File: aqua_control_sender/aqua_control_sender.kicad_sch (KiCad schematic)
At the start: 37 parts, among them J1 USB_C, J4 Conn_01x03, J5 Conn_01x03, SW1 RESET, SW2 BOOT, U1 ESP32-S3-WROOM-1, U2 LM1117-3.3, U3 RA-02_LORA

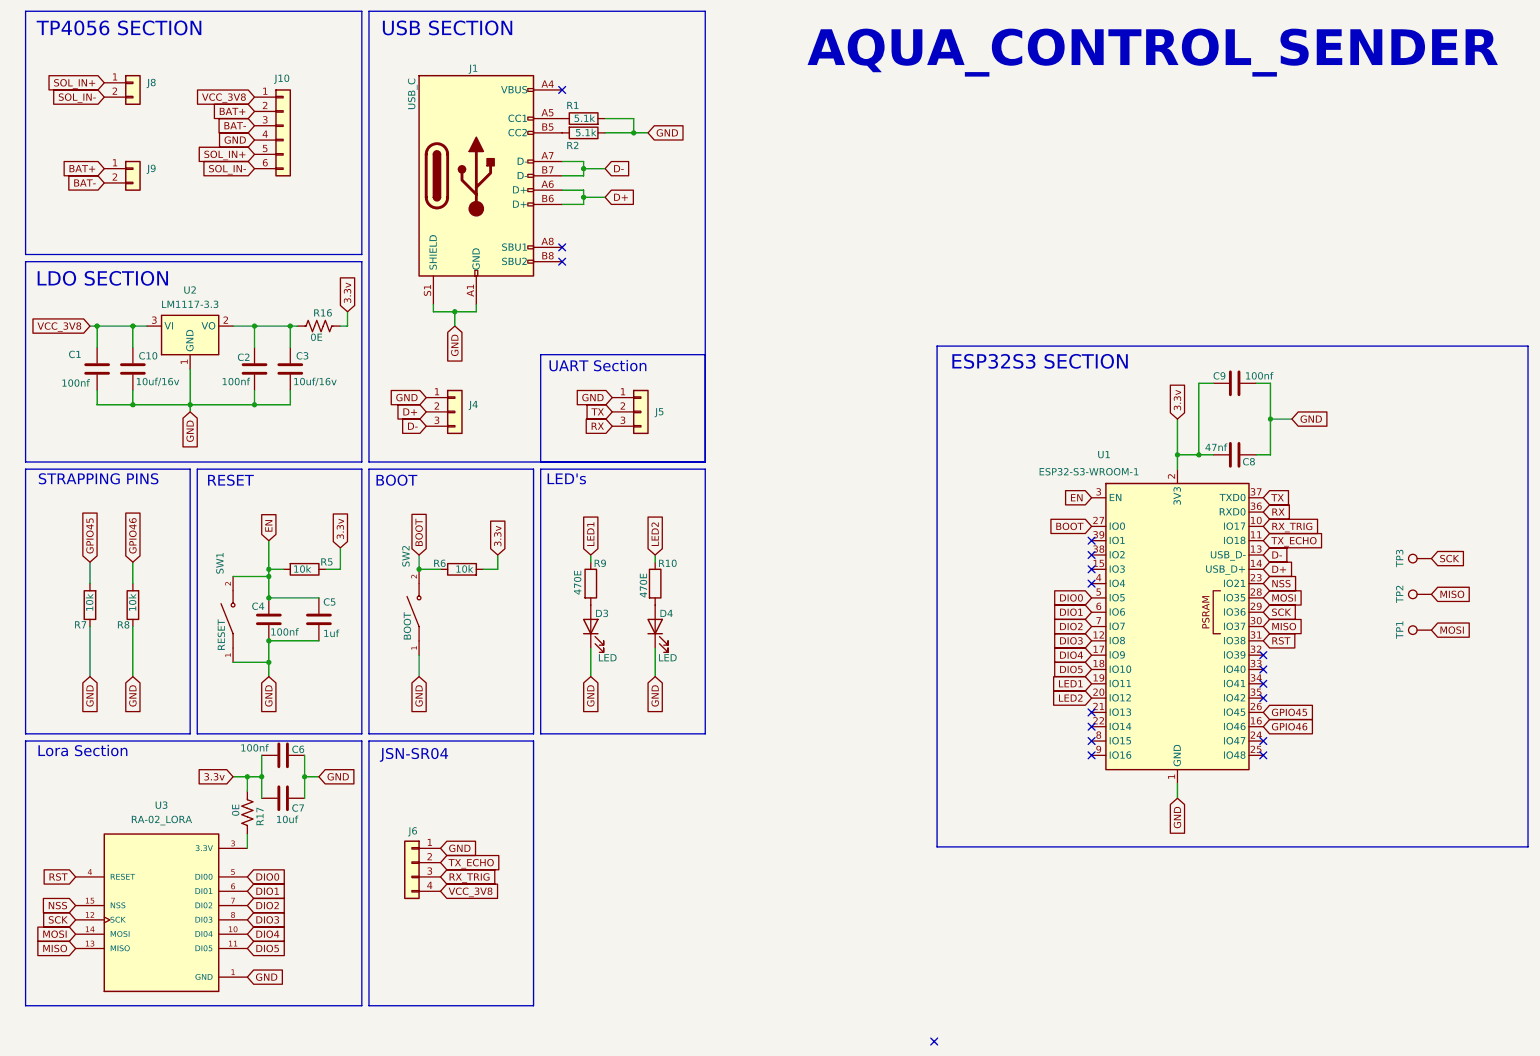
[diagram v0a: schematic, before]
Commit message: sender board complete
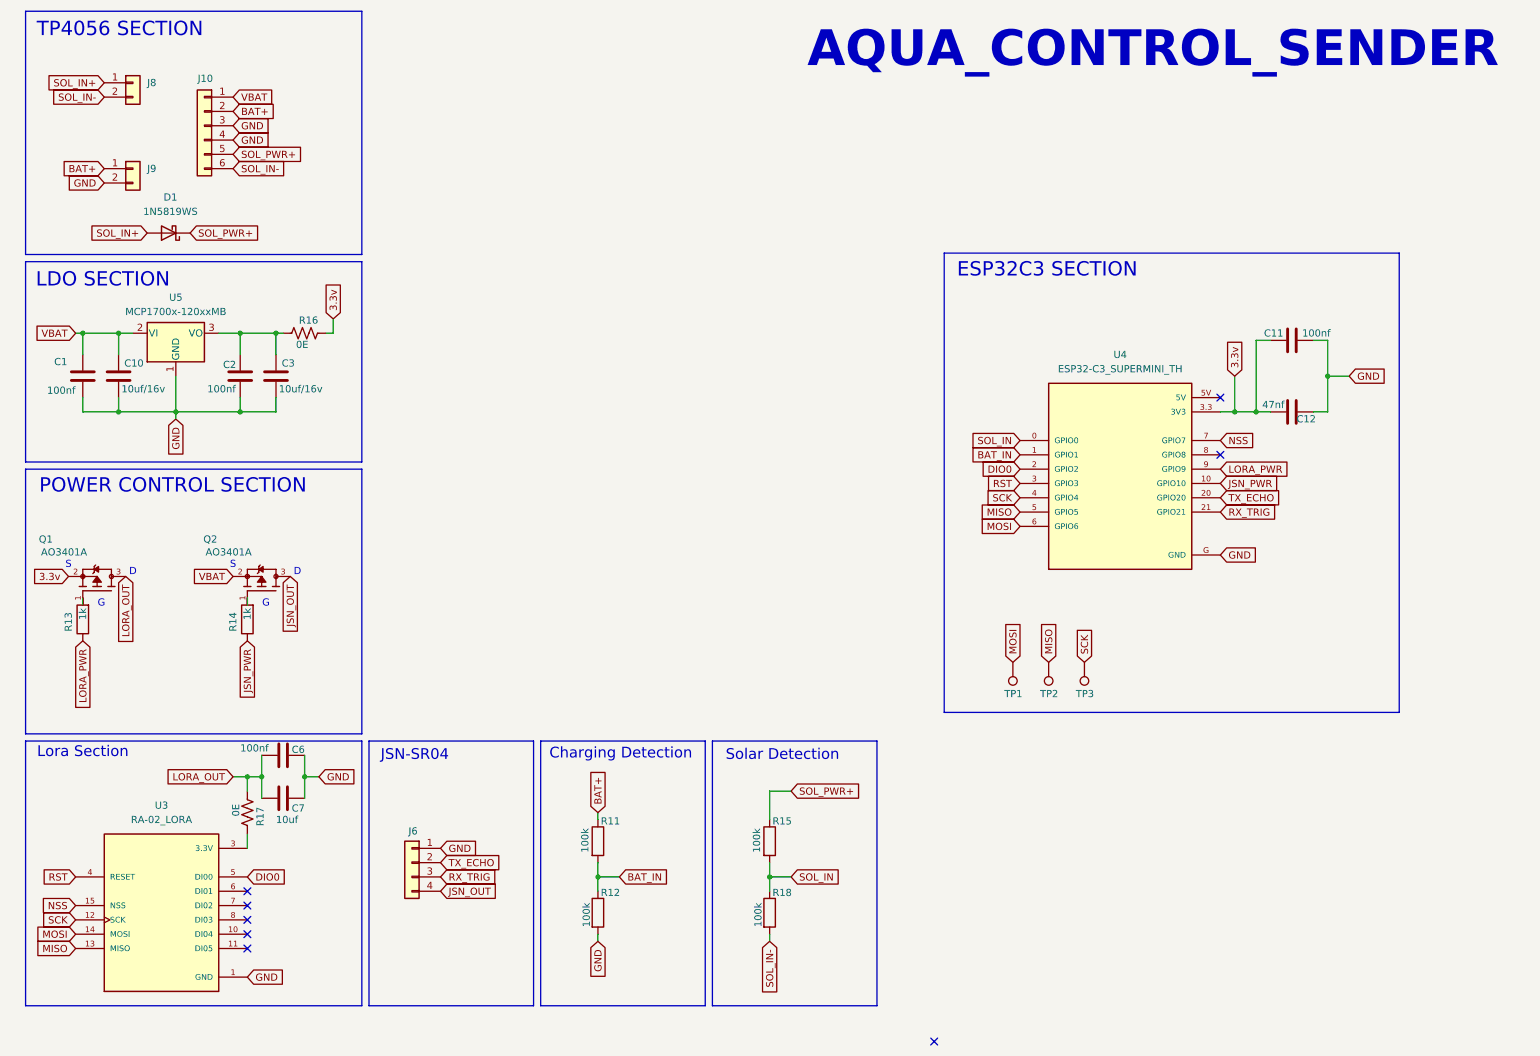
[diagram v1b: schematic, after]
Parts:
- removed C4, C9: 100nf, Capacitor_SMD:C_0805_2012Metric_Pad1.18x1.45mm_HandSolder, symbol Device:C
- removed C5: 1uf, Capacitor_SMD:C_0805_2012Metric_Pad1.18x1.45mm_HandSolder, symbol Device:C
- removed C8: 47nf, Capacitor_SMD:C_0805_2012Metric_Pad1.18x1.45mm_HandSolder, symbol Device:C
- removed D3, D4: LED, LED_SMD:LED_1206_3216Metric_Pad1.42x1.75mm_HandSolder, symbol Device:LED
- removed J1: USB_C, Connector_USB:USB_C_Receptacle_GCT_USB4110, symbol Connector:USB_C_Receptacle_USB2.0_16P
- removed J4, J5: Conn_01x03, Connector_PinSocket_2.54mm:PinSocket_1x03_P2.54mm_Vertical, symbol Connector_Generic:Conn_01x03
- removed R1, R2: 5.1k, Resistor_SMD:R_0805_2012Metric_Pad1.20x1.40mm_HandSolder, symbol Device:R
- removed R10, R9: 470E, Resistor_SMD:R_0805_2012Metric_Pad1.20x1.40mm_HandSolder, symbol Device:R
- removed R5, R6, R7, R8: 10k, Resistor_SMD:R_0805_2012Metric_Pad1.20x1.40mm_HandSolder, symbol Device:R
- removed SW1: RESET, Button_Switch_THT:SW_DIP_SPSTx01_Slide_6.7x4.1mm_W7.62mm_P2.54mm_LowProfile, symbol TS09-63-25-WT-160-SMT-TR:TS09-63-25-WT-160-SMT-TR
- removed SW2: BOOT, Button_Switch_THT:SW_DIP_SPSTx01_Slide_6.7x4.1mm_W7.62mm_P2.54mm_LowProfile, symbol TS09-63-25-WT-160-SMT-TR:TS09-63-25-WT-160-SMT-TR
- removed U1: ESP32-S3-WROOM-1, RF_Module:ESP32-S3-WROOM-1, symbol RF_Module:ESP32-S3-WROOM-1
- removed U2: LM1117-3.3, Package_TO_SOT_SMD:SOT-223-3_TabPin2, symbol Regulator_Linear:AMS1117-3.3
- added C11: 100nf, Capacitor_SMD:C_0805_2012Metric_Pad1.18x1.45mm_HandSolder, symbol Device:C
- added C12: 47nf, Capacitor_SMD:C_0805_2012Metric_Pad1.18x1.45mm_HandSolder, symbol Device:C
- added D1: 1N5819WS, Diode_SMD:D_SOD-323, symbol Diode:1N5819WS
- added Q1, Q2: AO3401A, mosfet:SOT23-3, symbol AO3401A:AO3401A
- added R11, R12, R15, R18: 100k, Resistor_SMD:R_0805_2012Metric_Pad1.20x1.40mm_HandSolder, symbol Device:R
- added R13, R14: 1k, Resistor_SMD:R_0805_2012Metric_Pad1.20x1.40mm_HandSolder, symbol Device:R
- added U4: ESP32-C3_SUPERMINI_TH, esp32c3:MODULE_ESP32-C3_SUPERMINI_TH, symbol ESP32-C3_SUPERMINI_TH:ESP32-C3_SUPERMINI_TH
- added U5: MCP1700x-120xxMB, Package_TO_SOT_SMD:SOT-89-3, symbol Regulator_Linear:MCP1700x-120xxMB
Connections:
- net BAT- is gone; now on net GND: J10.3 (Pin_3), J9.2 (Pin_2)
- net 3.3v: now also C11.1, C12.1, Q1.2, U4.3.3 (3V3); no longer C6.2, C7.2, R17.2
- net BAT+: now also R11.1
- net DIO0: now also U4.2 (GPIO2)
- net GND: now also C11.2, C12.2, R12.2, U4.G (GND), U5.1 (GND)
- net MISO: now also U4.5 (GPIO5)
- net MOSI: now also U4.6 (GPIO6)
- net NSS: now also U4.7 (GPIO7)
- net RST: now also U4.3 (GPIO3)
- net RX_TRIG: now also U4.21 (GPIO21)
- net SCK: now also U4.4 (GPIO4)
- net SOL_IN+: now also D1.2 (A); no longer J10.5 (Pin_5)
- net SOL_IN-: now also R18.2
- net TX_ECHO: now also U4.20 (GPIO20)
- net at C2.1, C3.1, R16.2: now also U5.3 (VO)
- net DIO1: no longer names the net of U3.6 (DI01)
- net DIO2: no longer names the net of U3.7 (DI02)
- net DIO3: no longer names the net of U3.8 (DI03)
- net DIO4: no longer names the net of U3.10 (DI04)
- net DIO5: no longer names the net of U3.11 (DI05)
- net VCC_3V8 renamed VBAT
- net VBAT: now also Q2.2, U5.2 (VI); no longer J6.4 (Pin_4)
- new net: Q1.1, R13.2
- new net: Q2.1, R14.2
- new net BAT_IN: R11.2, R12.1, U4.1 (GPIO1)
- new net JSN_OUT: J6.4 (Pin_4), Q2.3
- new net JSN_PWR: R14.1, U4.10 (GPIO10)
- new net LORA_OUT: C6.2, C7.2, Q1.3, R17.2
- new net LORA_PWR: R13.1, U4.9 (GPIO9)
- new net SOL_IN: R15.2, R18.1, U4.0 (GPIO0)
- new net SOL_PWR+: D1.1 (K), J10.5 (Pin_5), R15.1
- no-connect marks 18 -> 8
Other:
- note added: "Charging Detection"
- note added: "D"
- note added: "ESP32C3 SECTION"
- note added: "G"
- note added: "POWER CONTROL SECTION"
- note added: "S"
- note added: "Solar Detection"
- note removed: "BOOT"
- note removed: "ESP32S3 SECTION"
- note removed: "LED's"
- note removed: "RESET"
- note removed: "STRAPPING PINS"
- note removed: "UART Section"
- note removed: "USB SECTION"
- moved on the sheet: C1, C10, C2, C3, J10, R16

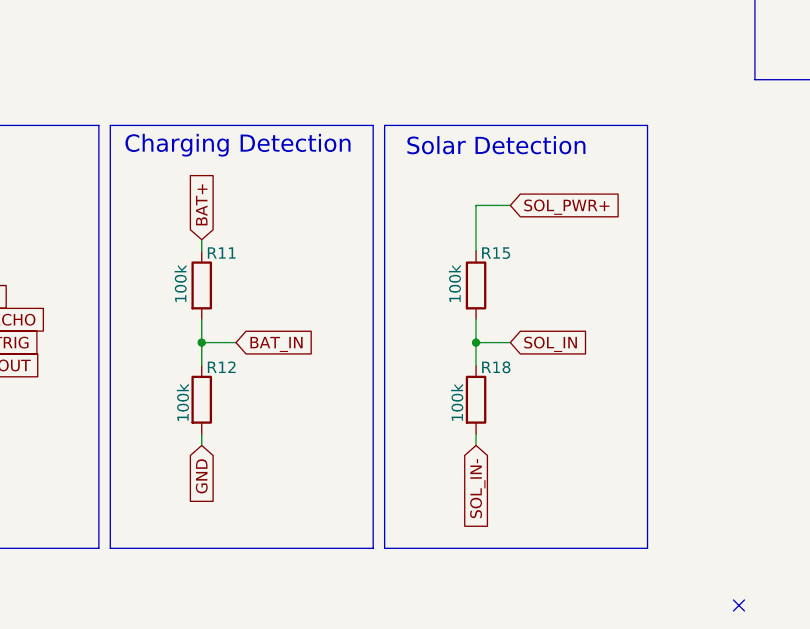
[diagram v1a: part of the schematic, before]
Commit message: final version
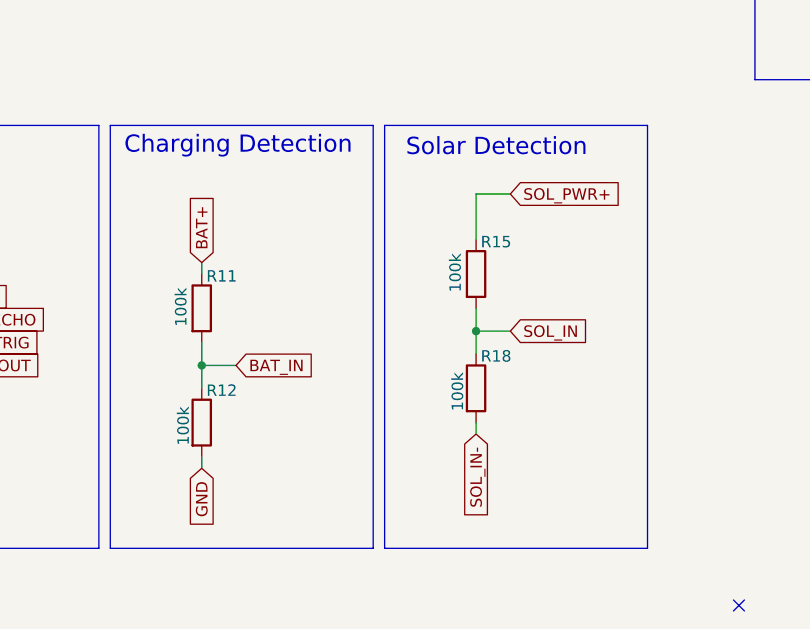
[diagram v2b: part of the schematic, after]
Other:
- moved on the sheet: R11, R12, R15, R18
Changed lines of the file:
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@@
 	)
 	(junction
-		(at 147.32 168.91)
+		(at 147.32 167.64)
 		(diameter 0)
 		(color 0 0 0 0)
@@
 	)
 	(junction
-		(at 116.84 168.91)
+		(at 116.84 171.45)
 		(diameter 0)
 		(color 0 0 0 0)
@@
 	(wire
 		(pts
-			(xy 116.84 168.91) (xy 116.84 171.45)
+			(xy 116.84 171.45) (xy 116.84 173.99)
 		)
 		(stroke
@@
 	(wire
 		(pts
-			(xy 116.84 179.07) (xy 116.84 180.34)
+			(xy 116.84 181.61) (xy 116.84 182.88)
 		)
 		(stroke
@@
 	(wire
 		(pts
-			(xy 151.13 153.67) (xy 147.32 153.67)
+			(xy 151.13 152.4) (xy 147.32 152.4)
 		)
 		(stroke
@@
 	(wire
 		(pts
-			(xy 120.65 168.91) (xy 116.84 168.91)
+			(xy 120.65 171.45) (xy 116.84 171.45)
 		)
 		(stroke
@@
 	(wire
 		(pts
-			(xy 116.84 158.75) (xy 116.84 157.48)
+			(xy 116.84 161.29) (xy 116.84 160.02)
 		)
 		(stroke
@@
 	(wire
 		(pts
-			(xy 147.32 179.07) (xy 147.32 180.34)
+			(xy 147.32 177.8) (xy 147.32 179.07)
 		)
 		(stroke
@@
 	(wire
 		(pts
-			(xy 116.84 166.37) (xy 116.84 168.91)
+			(xy 116.84 168.91) (xy 116.84 171.45)
 		)
 		(stroke
@@
 	(wire
 		(pts
-			(xy 147.32 166.37) (xy 147.32 168.91)
+			(xy 147.32 165.1) (xy 147.32 167.64)
 		)
 		(stroke
@@
 	(wire
 		(pts
-			(xy 147.32 153.67) (xy 147.32 158.75)
+			(xy 147.32 152.4) (xy 147.32 157.48)
 		)
 		(stroke
@@
 	(wire
 		(pts
-			(xy 147.32 168.91) (xy 147.32 171.45)
+			(xy 147.32 167.64) (xy 147.32 170.18)
 		)
 		(stroke
@@
 	(wire
 		(pts
-			(xy 151.13 168.91) (xy 147.32 168.91)
+			(xy 151.13 167.64) (xy 147.32 167.64)
 		)
 		(stroke
@@
 	(global_label "SOL_PWR+"
 		(shape input)
-		(at 151.13 153.67 0)
+		(at 151.13 152.4 0)
 		(fields_autoplaced yes)
 		(effects
@@
 		)
 		(property "Intersheetrefs" "${INTERSHEET_REFS}"
-			(at 164.2147 153.67 0)
+			(at 164.2147 152.4 0)
 			(hide yes)
 			(show_name no)
@@
 	(global_label "BAT_IN"
 		(shape input)
-		(at 120.65 168.91 0)
+		(at 120.65 171.45 0)
 		(fields_autoplaced yes)
 		(effects
@@
 		)
 		(property "Intersheetrefs" "${INTERSHEET_REFS}"
-			(at 129.8643 168.91 0)
+			(at 129.8643 171.45 0)
 			(hide yes)
 			(show_name no)
@@
 	(global_label "GND"
 		(shape input)
-		(at 116.84 180.34 270)
+		(at 116.84 182.88 270)
 		(fields_autoplaced yes)
 		(effects
@@
 		)
 		(property "Intersheetrefs" "${INTERSHEET_REFS}"
-			(at 116.84 187.1957 90)
+			(at 116.84 189.7357 90)
 			(hide yes)
 			(show_name no)
@@
 	(global_label "SOL_IN"
 		(shape input)
-		(at 151.13 168.91 0)
+		(at 151.13 167.64 0)
 		(fields_autoplaced yes)
 		(effects
@@
 		)
 		(property "Intersheetrefs" "${INTERSHEET_REFS}"
-			(at 160.5862 168.91 0)
+			(at 160.5862 167.64 0)
 			(hide yes)
 			(show_name no)
@@
 	(global_label "SOL_IN-"
 		(shape input)
-		(at 147.32 180.34 270)
+		(at 147.32 179.07 270)
 		(fields_autoplaced yes)
 		(effects
@@
 		)
 		(property "Intersheetrefs" "${INTERSHEET_REFS}"
-			(at 147.32 191.3686 90)
+			(at 147.32 190.0986 90)
 			(hide yes)
 			(show_name no)
@@
 	(global_label "BAT+"
 		(shape input)
-		(at 116.84 157.48 90)
+		(at 116.84 160.02 90)
 		(fields_autoplaced yes)
 		(effects
@@
 		)
 		(property "Intersheetrefs" "${INTERSHEET_REFS}"
-			(at 116.84 149.5962 90)
+			(at 116.84 152.1362 90)
 			(hide yes)
 			(show_name no)
@@
 	(symbol
 		(lib_id "Device:R")
-		(at 147.32 162.56 0)
+		(at 147.32 161.29 0)
 		(unit 1)
 		(body_style 1)
@@
 		(dnp no)
 		(property "Reference" "R15"
-			(at 147.828 159.004 0)
+			(at 147.828 157.734 0)
 			(show_name no)
 			(do_not_autoplace no)
@@
 		)
 		(property "Value" "100k"
-			(at 145.034 164.592 90)
+			(at 145.034 163.322 90)
 			(show_name no)
 			(do_not_autoplace no)
@@
 		)
 		(property "Footprint" "Resistor_SMD:R_0805_2012Metric_Pad1.20x1.40mm_HandSolder"
-			(at 145.542 162.56 90)
+			(at 145.542 161.29 90)
 			(hide yes)
 			(show_name no)
@@
 		)
 		(property "Datasheet" ""
-			(at 147.32 162.56 0)
+			(at 147.32 161.29 0)
 			(hide yes)
 			(show_name no)
@@
 		)
 		(property "Description" "Resistor"
-			(at 147.32 162.56 0)
+			(at 147.32 161.29 0)
 			(hide yes)
 			(show_name no)
@@
 	(symbol
 		(lib_id "Device:R")
-		(at 147.32 175.26 0)
+		(at 147.32 173.99 0)
 		(unit 1)
 		(body_style 1)
@@
 		(dnp no)
 		(property "Reference" "R18"
-			(at 147.828 171.704 0)
+			(at 147.828 170.434 0)
 			(show_name no)
 			(do_not_autoplace no)
@@
 		)
 		(property "Value" "100k"
-			(at 145.288 177.8 90)
+			(at 145.288 176.53 90)
 			(show_name no)
 			(do_not_autoplace no)
@@
 		)
 		(property "Footprint" "Resistor_SMD:R_0805_2012Metric_Pad1.20x1.40mm_HandSolder"
-			(at 145.542 175.26 90)
+			(at 145.542 173.99 90)
 			(hide yes)
 			(show_name no)
@@
 		)
 		(property "Datasheet" ""
-			(at 147.32 175.26 0)
+			(at 147.32 173.99 0)
 			(hide yes)
 			(show_name no)
@@
 		)
 		(property "Description" "Resistor"
-			(at 147.32 175.26 0)
+			(at 147.32 173.99 0)
 			(hide yes)
 			(show_name no)
@@
 	(symbol
 		(lib_id "Device:R")
-		(at 116.84 162.56 0)
+		(at 116.84 165.1 0)
 		(unit 1)
 		(body_style 1)
@@
 		(dnp no)
 		(property "Reference" "R11"
-			(at 117.348 159.004 0)
+			(at 117.348 161.544 0)
 			(show_name no)
 			(do_not_autoplace no)
@@
 		)
 		(property "Value" "100k"
-			(at 114.554 164.592 90)
+			(at 114.554 167.132 90)
 			(show_name no)
 			(do_not_autoplace no)
@@
 		)
 		(property "Footprint" "Resistor_SMD:R_0805_2012Metric_Pad1.20x1.40mm_HandSolder"
-			(at 115.062 162.56 90)
+			(at 115.062 165.1 90)
 			(hide yes)
 			(show_name no)
@@
 		)
 		(property "Datasheet" ""
-			(at 116.84 162.56 0)
+			(at 116.84 165.1 0)
 			(hide yes)
 			(show_name no)
@@
 		)
 		(property "Description" "Resistor"
-			(at 116.84 162.56 0)
+			(at 116.84 165.1 0)
 			(hide yes)
 			(show_name no)
@@
 	(symbol
 		(lib_id "Device:R")
-		(at 116.84 175.26 0)
+		(at 116.84 177.8 0)
 		(unit 1)
 		(body_style 1)
@@
 		(dnp no)
 		(property "Reference" "R12"
-			(at 117.348 171.704 0)
+			(at 117.348 174.244 0)
 			(show_name no)
 			(do_not_autoplace no)
@@
 		)
 		(property "Value" "100k"
-			(at 114.808 177.8 90)
+			(at 114.808 180.34 90)
 			(show_name no)
 			(do_not_autoplace no)
@@
 		)
 		(property "Footprint" "Resistor_SMD:R_0805_2012Metric_Pad1.20x1.40mm_HandSolder"
-			(at 115.062 175.26 90)
+			(at 115.062 177.8 90)
 			(hide yes)
 			(show_name no)
@@
 		)
 		(property "Datasheet" ""
-			(at 116.84 175.26 0)
+			(at 116.84 177.8 0)
 			(hide yes)
 			(show_name no)
@@
 		)
 		(property "Description" "Resistor"
-			(at 116.84 175.26 0)
+			(at 116.84 177.8 0)
 			(hide yes)
 			(show_name no)
